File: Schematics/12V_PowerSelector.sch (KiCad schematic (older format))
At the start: 3 parts

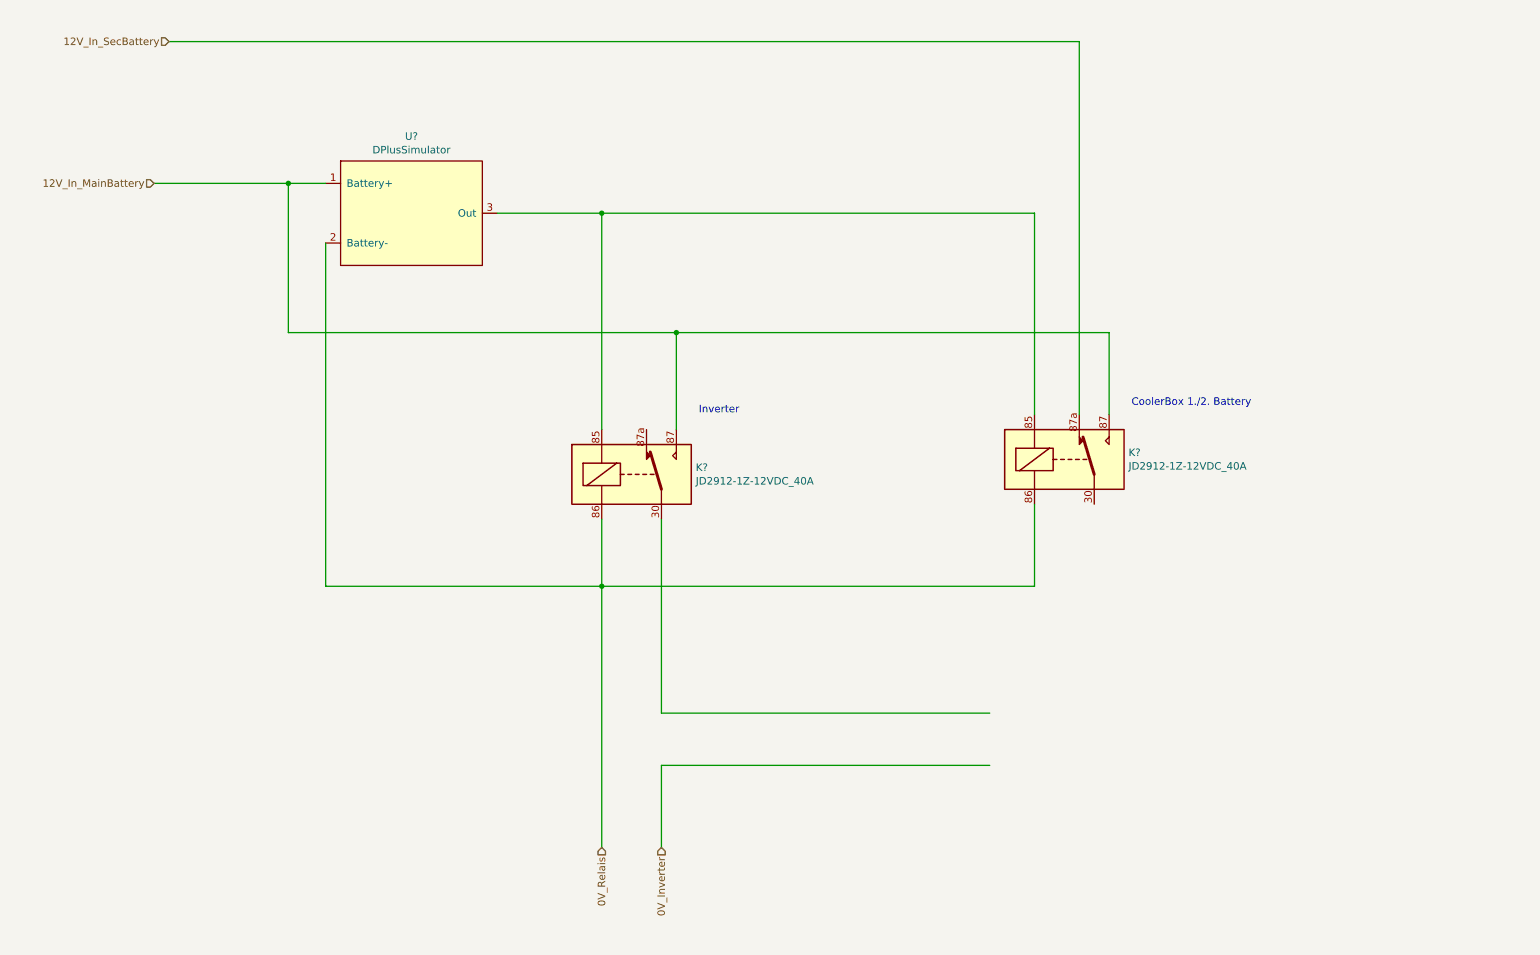
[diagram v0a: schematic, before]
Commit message: Finalize Schematic
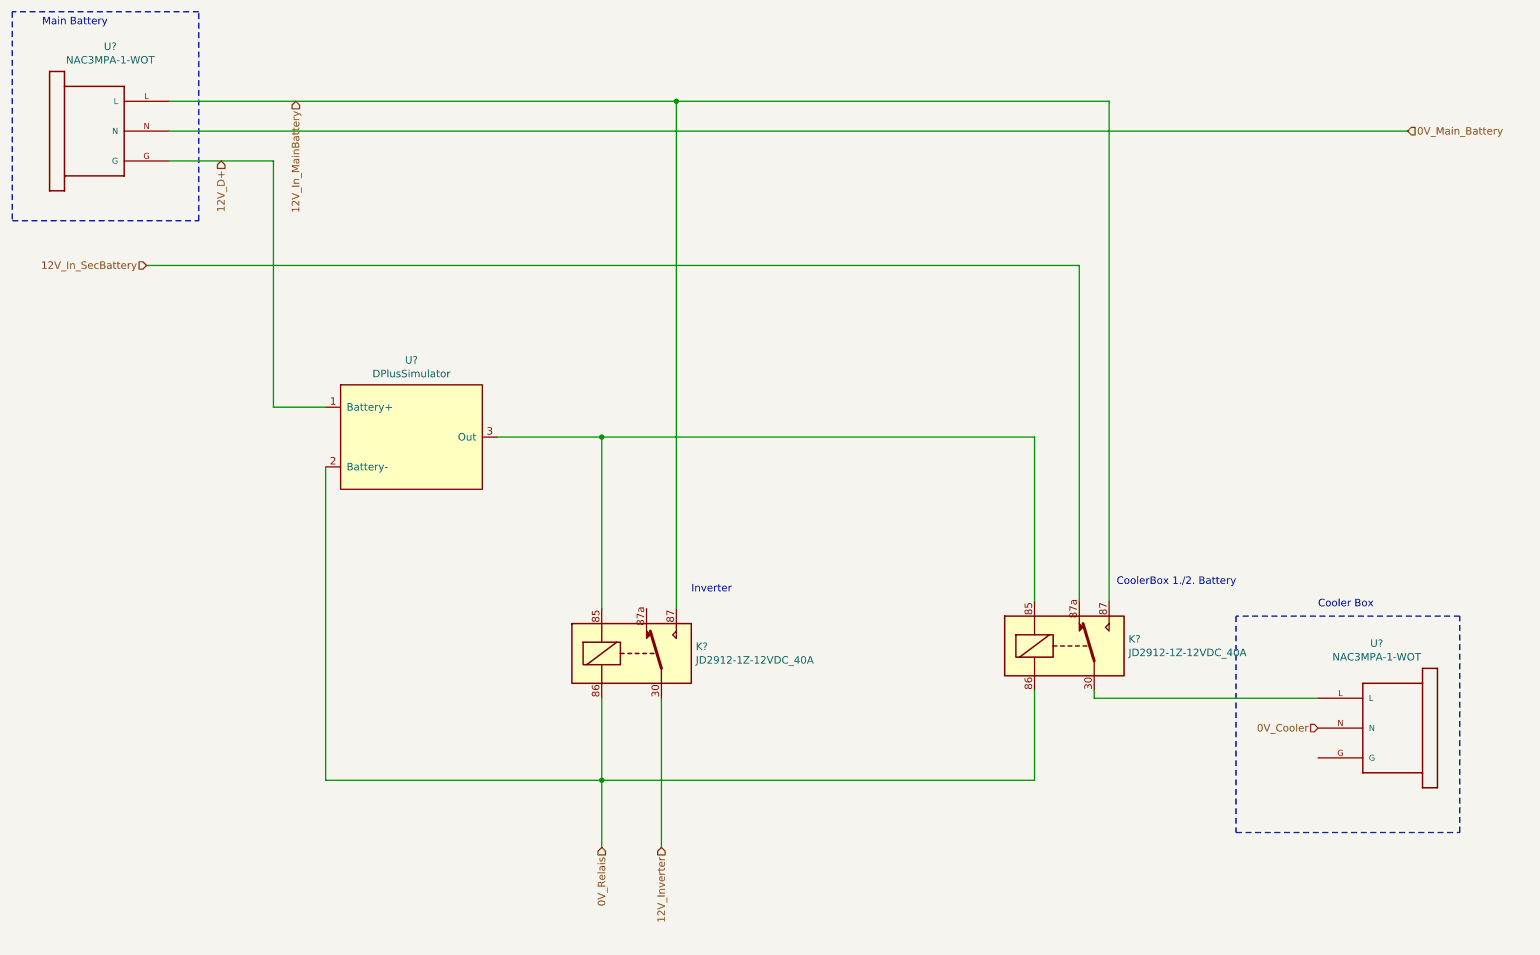
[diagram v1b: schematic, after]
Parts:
- added U? (x2): NAC3MPA-1-WOT, NAC3MPA-1-WOT, symbol BatteryBox-rescue:NAC3MPA-1-WOT-NAC3MPA-1-WOT
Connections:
- net labels added: 0V_Cooler, 0V_Main_Battery, 12V_D+, 12V_Inverter
- net labels removed: 0V_Inverter
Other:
- note added: "Cooler Box"
- note added: "Main Battery"
- moved on the sheet: K?, U?
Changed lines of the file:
@@
 L MyParts:DPlusSimulator U?
 U 1 1 60D69C17
-P 2850 2250
+P 2850 3750
 AR Path="/5F0EC429/60D69C17" Ref="U?"  Part="1"
 AR Path="/60D529AB/60D52DDD/60D69C17" Ref="U?"  Part="1"
-F 0 "U?" H 3325 3115 50  0000 C CNN
-F 1 "DPlusSimulator" H 3325 3024 50  0000 C CNN
-F 2 "" H 4000 2850 50  0001 C CNN
-F 3 "" H 4000 2850 50  0001 C CNN
-	1    2850 2250
+F 0 "U?" H 3325 4615 50  0000 C CNN
+F 1 "DPlusSimulator" H 3325 4524 50  0000 C CNN
+F 2 "" H 4000 4350 50  0001 C CNN
+F 3 "" H 4000 4350 50  0001 C CNN
+	1    2850 3750
 	1    0    0    -1
 $EndComp
-Text HLabel 1600 1700 0    50   Input ~ 0
+Text HLabel 2550 1150 3    50   Input ~ 0
 12V_In_MainBattery
-Wire Wire Line
-	1600 1700 2500 1700
-Wire Wire Line
-	2500 1700 2500 2700
-Connection ~ 2500 1700
-Wire Wire Line
-	2500 1700 2750 1700
-Text HLabel 1700 750  0    50   Input ~ 0
+Text HLabel 1550 2250 0    50   Input ~ 0
 12V_In_SecBattery
 Wire Wire Line
-	5000 5250 7200 5250
-Wire Wire Line
-	7200 5600 5000 5600
-Wire Wire Line
-	2750 2100 2750 4400
-Wire Wire Line
-	5000 5600 5000 6150
-Text Notes 5250 3250 0    50   ~ 0
+	2750 3600 2750 5700
+Text Notes 5200 4450 0    50   ~ 0
 Inverter
-Text Notes 8150 3200 0    50   ~ 0
+Text Notes 8050 4400 0    50   ~ 0
 CoolerBox 1./2. Battery
-Connection ~ 5100 2700
-Wire Wire Line
-	2500 2700 5100 2700
-Wire Wire Line
-	5100 2700 5100 3350
-Wire Wire Line
-	5000 3950 5000 5250
 $Comp
 L MyParts:JD2912-1Z-12VDC_40A K?
 U 1 1 60D69C1D
-P 4800 3650
+P 4800 4850
 AR Path="/5F0EC429/60D69C1D" Ref="K?"  Part="1"
 AR Path="/60D529AB/60D52DDD/60D69C1D" Ref="K?"  Part="1"
-F 0 "K?" H 5230 3696 50  0000 L CNN
-F 1 "JD2912-1Z-12VDC_40A" H 5230 3605 50  0000 L CNN
-F 2 "Relay_THT:Relay_StandexMeder_DIP_LowProfile" H 5250 3600 50  0001 L CNN
-F 3 "https://standexelectronics.com/wp-content/uploads/datasheet_reed_relay_DIP.pdf" H 4800 3650 50  0001 C CNN
-	1    4800 3650
+F 0 "K?" H 5230 4896 50  0000 L CNN
+F 1 "JD2912-1Z-12VDC_40A" H 5230 4805 50  0000 L CNN
+F 2 "Relay_THT:Relay_StandexMeder_DIP_LowProfile" H 5250 4800 50  0001 L CNN
+F 3 "https://standexelectronics.com/wp-content/uploads/datasheet_reed_relay_DIP.pdf" H 4800 4850 50  0001 C CNN
+	1    4800 4850
 	1    0    0    -1
 $EndComp
@@
 L MyParts:JD2912-1Z-12VDC_40A K?
 U 1 1 60D6EC93
-P 7700 3550
+P 7700 4800
 AR Path="/5F0EC429/60D6EC93" Ref="K?"  Part="1"
 AR Path="/60D529AB/60D52DDD/60D6EC93" Ref="K?"  Part="1"
-F 0 "K?" H 8130 3596 50  0000 L CNN
-F 1 "JD2912-1Z-12VDC_40A" H 8130 3505 50  0000 L CNN
-F 2 "Relay_THT:Relay_StandexMeder_DIP_LowProfile" H 8150 3500 50  0001 L CNN
-F 3 "https://standexelectronics.com/wp-content/uploads/datasheet_reed_relay_DIP.pdf" H 7700 3550 50  0001 C CNN
-	1    7700 3550
+F 0 "K?" H 8130 4846 50  0000 L CNN
+F 1 "JD2912-1Z-12VDC_40A" H 8130 4755 50  0000 L CNN
+F 2 "Relay_THT:Relay_StandexMeder_DIP_LowProfile" H 8150 4750 50  0001 L CNN
+F 3 "https://standexelectronics.com/wp-content/uploads/datasheet_reed_relay_DIP.pdf" H 7700 4800 50  0001 C CNN
+	1    7700 4800
 	1    0    0    -1
 $EndComp
 Wire Wire Line
-	7500 1900 7500 3250
+	7500 3400 7500 4500
 Wire Wire Line
-	8000 2700 8000 3250
+	3900 3400 4600 3400
+Connection ~ 4600 3400
 Wire Wire Line
-	7800 750  7800 3250
+	4600 3400 7500 3400
 Wire Wire Line
-	5100 2700 8000 2700
+	4600 4550 4600 3400
 Wire Wire Line
-	1700 750  7800 750
+	4600 5150 4600 5700
 Wire Wire Line
-	3900 1900 4600 1900
-Connection ~ 4600 1900
+	4600 5700 7500 5700
 Wire Wire Line
-	4600 1900 7500 1900
+	7500 5700 7500 5100
+Connection ~ 4600 5700
 Wire Wire Line
-	4600 3350 4600 1900
+	4600 5700 4600 6150
 Wire Wire Line
-	4600 3950 4600 4400
-Wire Wire Line
-	4600 4400 7500 4400
-Wire Wire Line
-	7500 4400 7500 3850
-Connection ~ 4600 4400
-Wire Wire Line
-	4600 4400 4600 6150
-Wire Wire Line
-	2750 4400 4600 4400
+	2750 5700 4600 5700
 Text HLabel 5000 6150 3    50   Input ~ 0
-0V_Inverter
+12V_Inverter
 Text HLabel 4600 6150 3    50   Input ~ 0
 0V_Relais
+Wire Wire Line
+	5000 5150 5000 6150
+$Comp
+L BatteryBox-rescue:NAC3MPA-1-WOT-NAC3MPA-1-WOT U?
+U 1 1 60D6EF2E
+P 9600 5550
+AR Path="/5F0C81D9/60D6EF2E" Ref="U?"  Part="1"
+AR Path="/60D529AB/60D84F6F/60D6EF2E" Ref="U?"  Part="1"
+AR Path="/60D529AB/60D52DDD/60D6EF2E" Ref="U?"  Part="1"
+F 0 "U?" H 9407 6317 50  0000 C CNN
+F 1 "NAC3MPA-1-WOT" H 9407 6226 50  0000 C CNN
+F 2 "NAC3MPA-1-WOT" H 9600 5550 50  0001 L BNN
+F 3 "" H 9600 5550 50  0001 C CNN
+	1    9600 5550
+	-1   0    0    -1
+$EndComp
+Wire Wire Line
+	7900 5150 9400 5150
+Wire Wire Line
+	2400 3200 2750 3200
+Text HLabel 2050 1550 3    50   Input ~ 0
+12V_D+
+Text HLabel 9400 5350 0    50   Input ~ 0
+0V_Cooler
+Wire Notes Line
+	8850 4600 8850 6050
+Wire Notes Line
+	8850 6050 10350 6050
+Wire Notes Line
+	10350 6050 10350 4600
+Wire Notes Line
+	10350 4600 8850 4600
+Text Notes 9400 4550 0    50   ~ 0
+Cooler Box
+Wire Wire Line
+	7900 5100 7900 5150
+$Comp
+L BatteryBox-rescue:NAC3MPA-1-WOT-NAC3MPA-1-WOT U?
+U 1 1 60D75CC0
+P 1500 1550
+AR Path="/5F0C81D9/60D75CC0" Ref="U?"  Part="1"
+AR Path="/60D529AB/60D84F6F/60D75CC0" Ref="U?"  Part="1"
+AR Path="/60D529AB/60D52DDD/60D75CC0" Ref="U?"  Part="1"
+F 0 "U?" H 1307 2317 50  0000 C CNN
+F 1 "NAC3MPA-1-WOT" H 1307 2226 50  0000 C CNN
+F 2 "NAC3MPA-1-WOT" H 1500 1550 50  0001 L BNN
+F 3 "" H 1500 1550 50  0001 C CNN
+	1    1500 1550
+	1    0    0    -1
+$EndComp
+Wire Wire Line
+	2400 3200 2400 1550
+Wire Wire Line
+	2400 1550 1700 1550
+Wire Wire Line
+	1700 1150 5100 1150
+Wire Wire Line
+	1700 1350 10000 1350
+Text HLabel 10000 1350 2    50   Input ~ 0
+0V_Main_Battery
+Wire Wire Line
+	1550 2250 7800 2250
+Wire Wire Line
+	5100 4550 5100 1150
+Connection ~ 5100 1150
+Wire Wire Line
+	8000 1150 8000 4500
+Wire Wire Line
+	5100 1150 8000 1150
+Wire Wire Line
+	7800 4500 7800 2250
+Wire Notes Line
+	650  550  650  1950
+Wire Notes Line
+	650  1950 1900 1950
+Wire Notes Line
+	1900 1950 1900 550
+Wire Notes Line
+	1900 550  650  550
+Text Notes 850  650  0    50   ~ 0
+Main Battery
 $EndSCHEMATC
